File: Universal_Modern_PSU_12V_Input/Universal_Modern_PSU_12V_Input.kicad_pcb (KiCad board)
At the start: 2 copper layers, 70 x 50 mm, 24 parts, among them J1 +12VDC Input, J2 Power Output, Q1 SUP53P06-20-E3, U1 DFR0831, U2 NKE1212SC, U3 R-78CK5.0-0.5

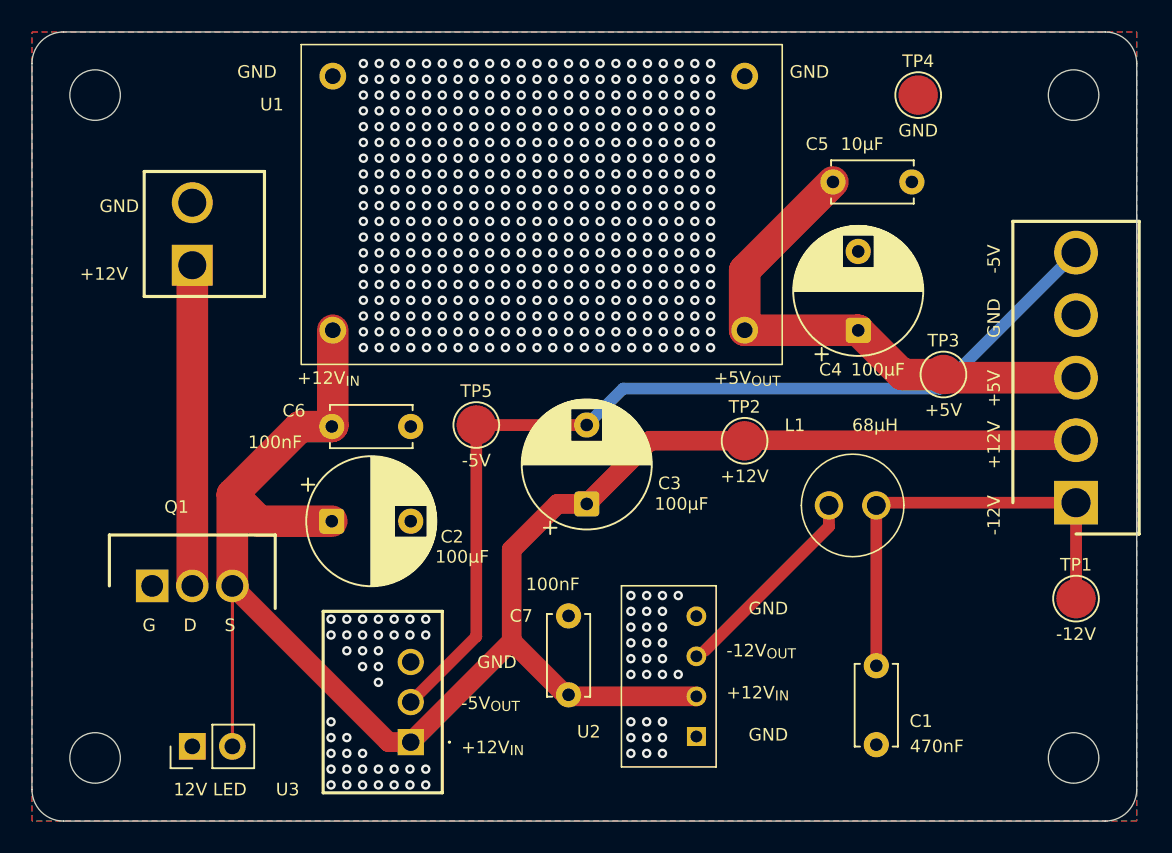
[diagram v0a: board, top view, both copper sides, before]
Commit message: Further refinements to PCB layout
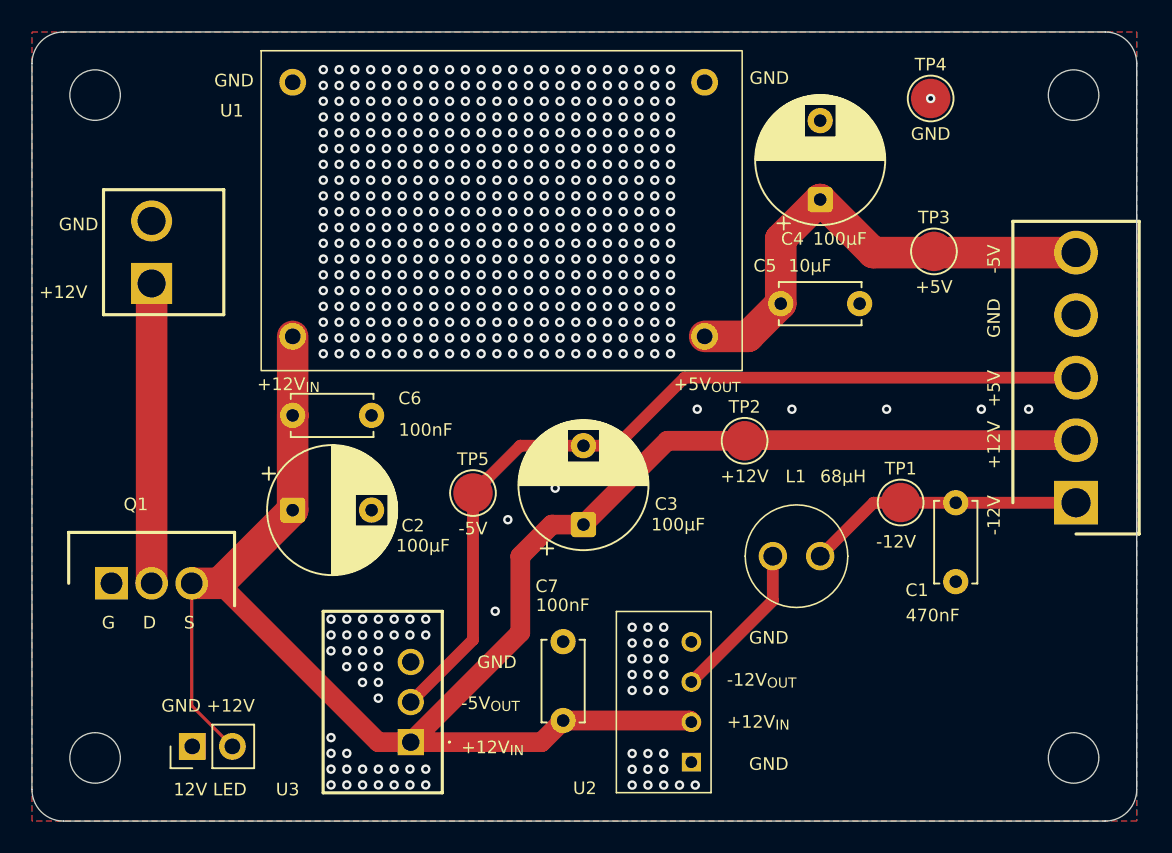
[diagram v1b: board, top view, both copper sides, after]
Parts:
- moved TP1 12.7 mm to (161.1, 108.3)
- moved C1 11.5 mm to (164.6, 113.3)
- moved C4 8.63 mm to (156.0, 89.1)
- moved C5 8.39 mm to (158.5, 95.7)
- moved TP3 7.82 mm to (163.2, 92.4)
- moved L1 4.79 mm to (156.0, 111.7)
- moved TP5 4.32 mm to (134.0, 107.7)
- moved J1 2.83 mm to (113.6, 94.4)
- moved Q1 2.58 mm to (111.1, 113.4)
- moved C2 2.58 mm to (122.6, 108.8)
- moved C6 2.58 mm to (122.6, 102.8)
- moved U1 2.57 mm to (134.0, 77.9)
- moved C7 1.67 mm to (139.7, 117.1)
- moved U2 1.66 mm to (147.8, 124.8)
- moved C3 1.33 mm to (141.0, 109.7)
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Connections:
- J2 pad 3: /+5V_{OUT} -> /-5V_{OUT}
- J2 pad 5: /-5V_{OUT} -> /+5V_{OUT}
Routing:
- net /-12V_{OUT}: track 29.0 -> 17.6 mm
- net /-5V_{OUT}: track 61.8 -> 56.1 mm
- net /+5V_{OUT}: track 34.0 -> 30.9 mm
- net /-12V: track 12.5 -> 10.1 mm
- net /+12V_{IN}: track 120.3 -> 118.3 mm
- net /+12V_{SUPPLY}: track 20.3 -> 19.0 mm
- net /GND: vias 506 -> 513
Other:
- board text added: "GND +12V"
